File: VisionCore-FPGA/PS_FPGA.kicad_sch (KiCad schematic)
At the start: 1 part, among them U1 Zynq 7000 - XCZU4EV

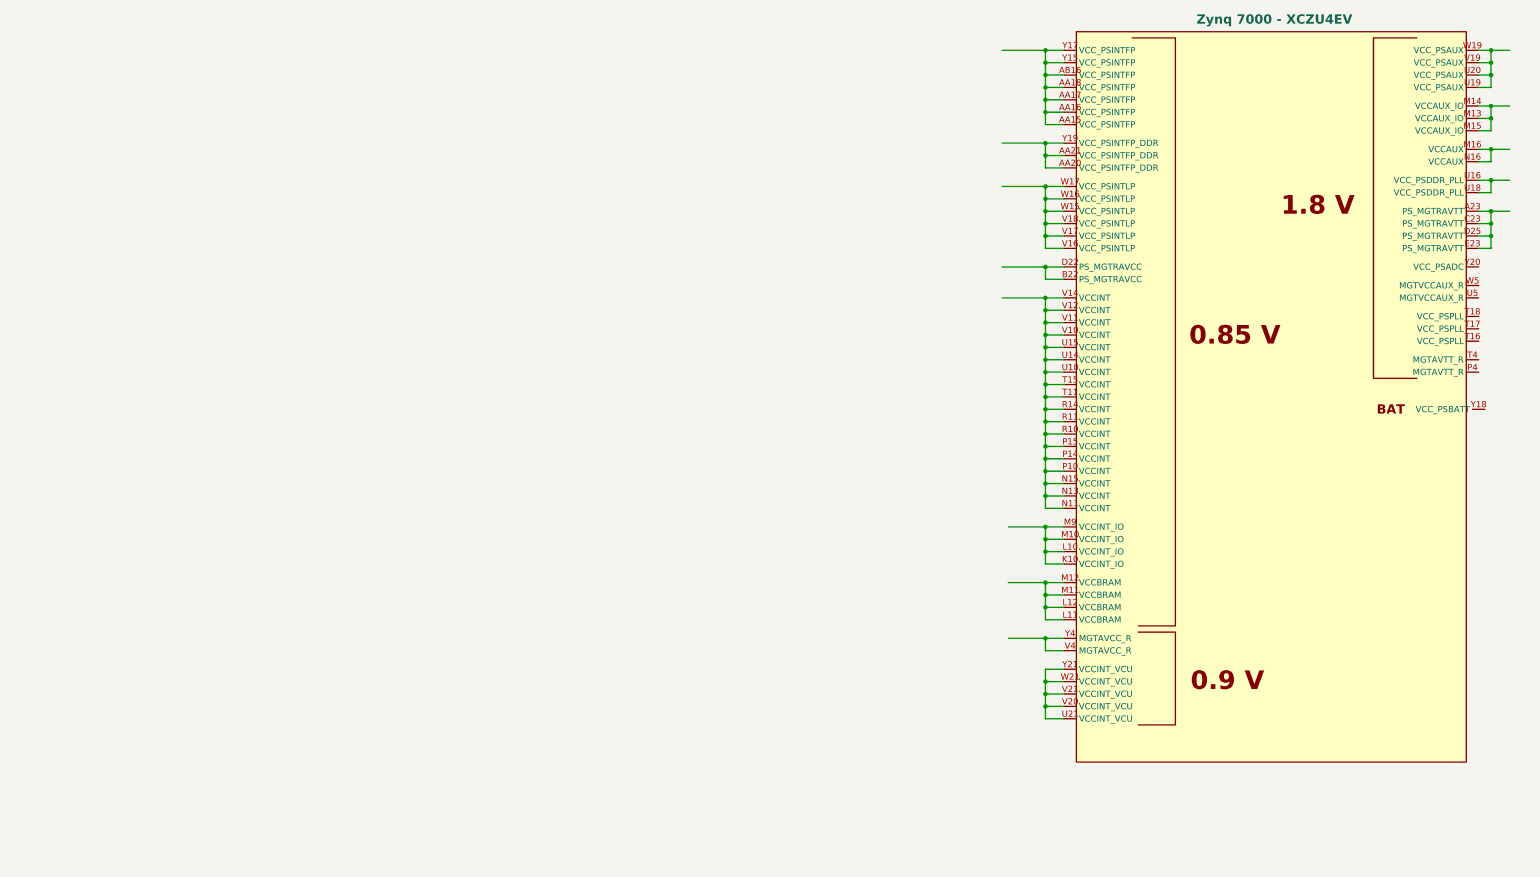
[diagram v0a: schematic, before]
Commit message: Added some net color filtering
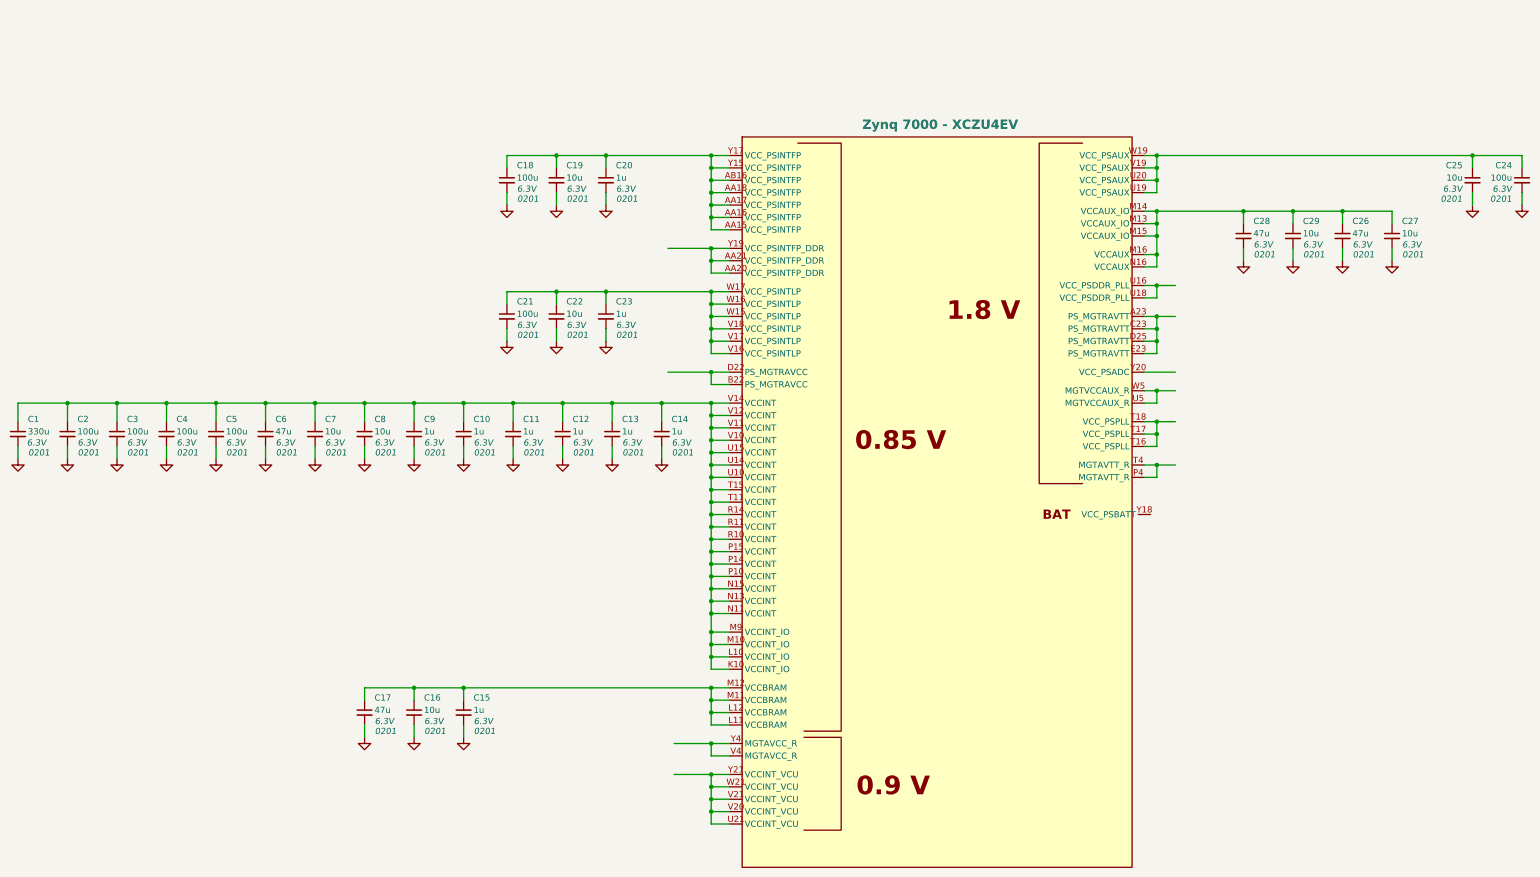
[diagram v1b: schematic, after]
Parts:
- added C1: 330u, symbol Device:C_Small
- added C10, C11, C12, C13, C14, C15, C20, C23, C9: 1u, symbol Device:C_Small
- added C16, C19, C22, C25, C27, C29, C7, C8: 10u, symbol Device:C_Small
- added C17, C26, C28, C6: 47u, symbol Device:C_Small
- added C18, C2, C21, C24, C3, C4, C5: 100u, symbol Device:C_Small
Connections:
- net at U1.AA15 (VCC_PSINTFP), U1.AA16 (VCC_PSINTFP), U1.AA17 (VCC_PSINTFP)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: now also C18.1, C19.1, C20.1
- net at U1.K10 (VCCINT_IO), U1.L10 (VCCINT_IO), U1.M10 (VCCINT_IO)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: now also U1.N11 (VCCINT), U1.N13 (VCCINT), U1.N15 (VCCINT), U1.P10 (VCCINT), U1.P14 (VCCINT), U1.P15 (VCCINT), U1.R10 (VCCINT), U1.R11 (VCCINT), U1.R14 (VCCINT), U1.T11 (VCCINT), U1.T15 (VCCINT), U1.U10 (VCCINT), U1.U14 (VCCINT), U1.U15 (VCCINT), U1.V10 (VCCINT), U1.V11 (VCCINT), U1.V12 (VCCINT), U1.V14 (VCCINT), C1.1, C10.1, C11.1, C12.1, C13.1, C14.1, C2.1, C3.1, C4.1, C5.1, C6.1, C7.1, C8.1, C9.1
- net at U1.L11 (VCCBRAM), U1.L12 (VCCBRAM), U1.M11 (VCCBRAM)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: now also C15.1, C16.1, C17.1
- net at U1.M13 (VCCAUX_IO), U1.M14 (VCCAUX_IO), U1.M15 (VCCAUX_IO): now also U1.M16 (VCCAUX), U1.N16 (VCCAUX), C26.1, C27.1, C28.1, C29.1
- net at U1.P4 (MGTAVTT_R): now also U1.T4 (MGTAVTT_R)
- net at U1.T16 (VCC_PSPLL): now also U1.T17 (VCC_PSPLL), U1.T18 (VCC_PSPLL)
- net at U1.U19 (VCC_PSAUX), U1.U20 (VCC_PSAUX), U1.V19 (VCC_PSAUX)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: now also C24.1, C25.1
- net at U1.U5 (MGTVCCAUX_R): now also U1.W5 (MGTVCCAUX_R)
- net at U1.V16 (VCC_PSINTLP), U1.V17 (VCC_PSINTLP), U1.V18 (VCC_PSINTLP)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: now also C21.1, C22.1, C23.1
- new net GND: C1.2, C10.2, C11.2, C12.2, C13.2, C14.2, C15.2, C16.2, C17.2, C18.2, C19.2, C2.2, C20.2, C21.2, C22.2, C23.2, C24.2, C25.2, C26.2, C27.2, C28.2, C29.2, C3.2, C4.2, C5.2, C6.2, C7.2, C8.2, C9.2
